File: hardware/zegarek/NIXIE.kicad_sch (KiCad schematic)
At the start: 42 parts, among them M1 74141DIP16, M2 74141DIP16, M3 74141DIP16, M4 74141DIP16, U5 SN74LVC8T245, U6 SN74LVC8T245

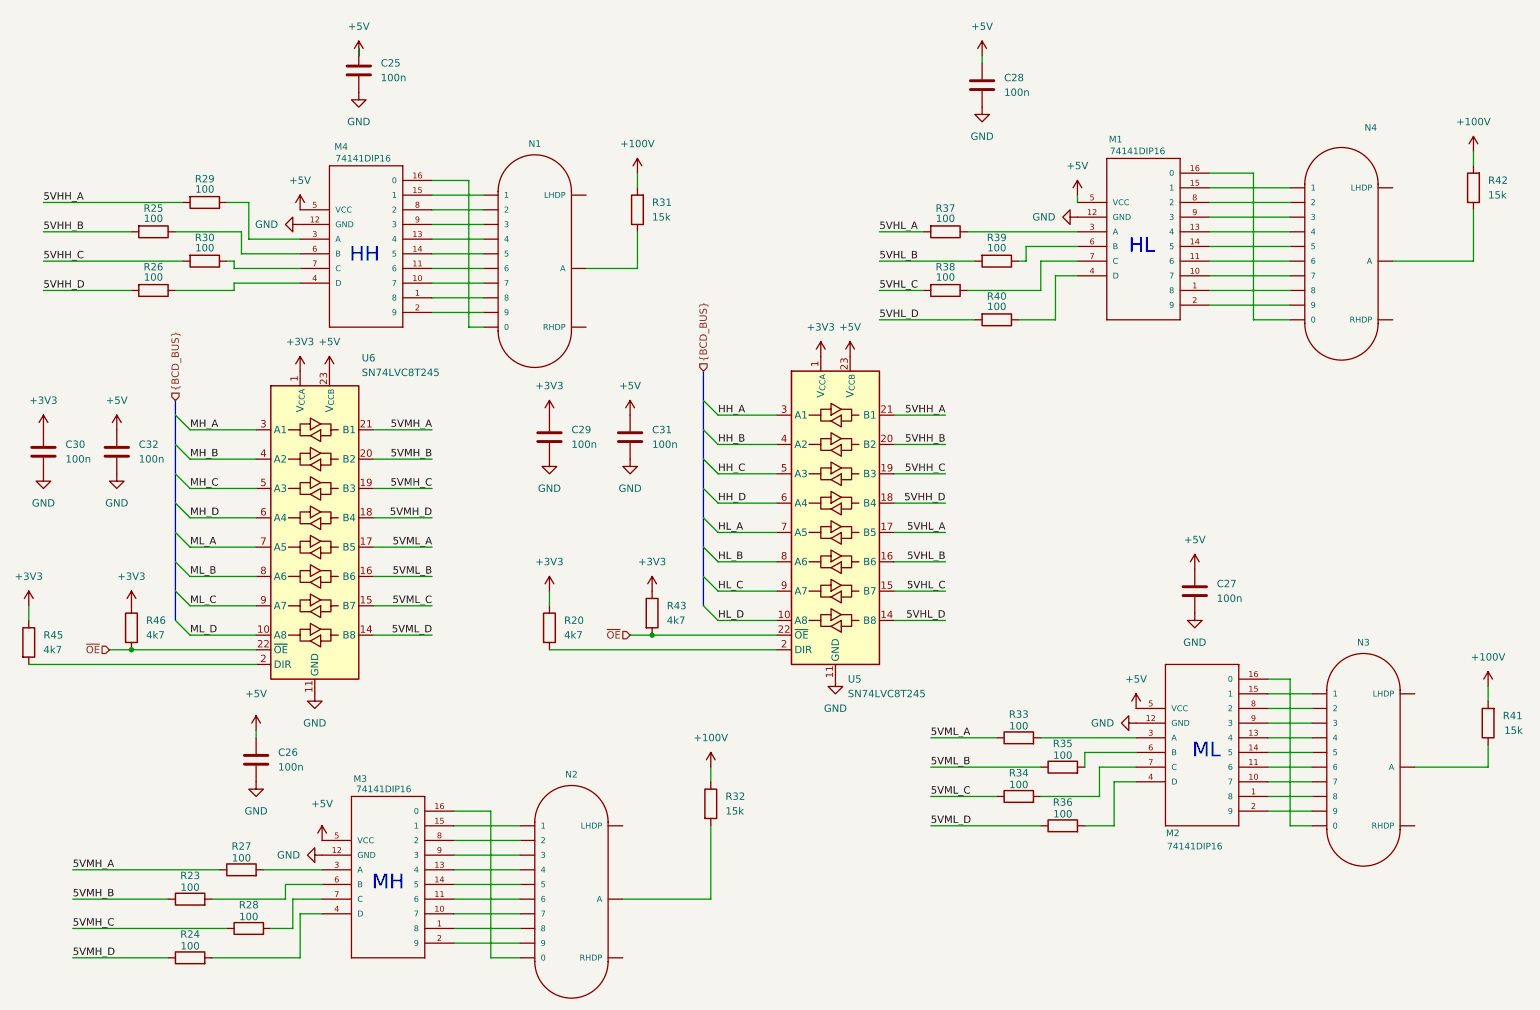
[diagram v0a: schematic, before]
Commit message: reqenerating postprod
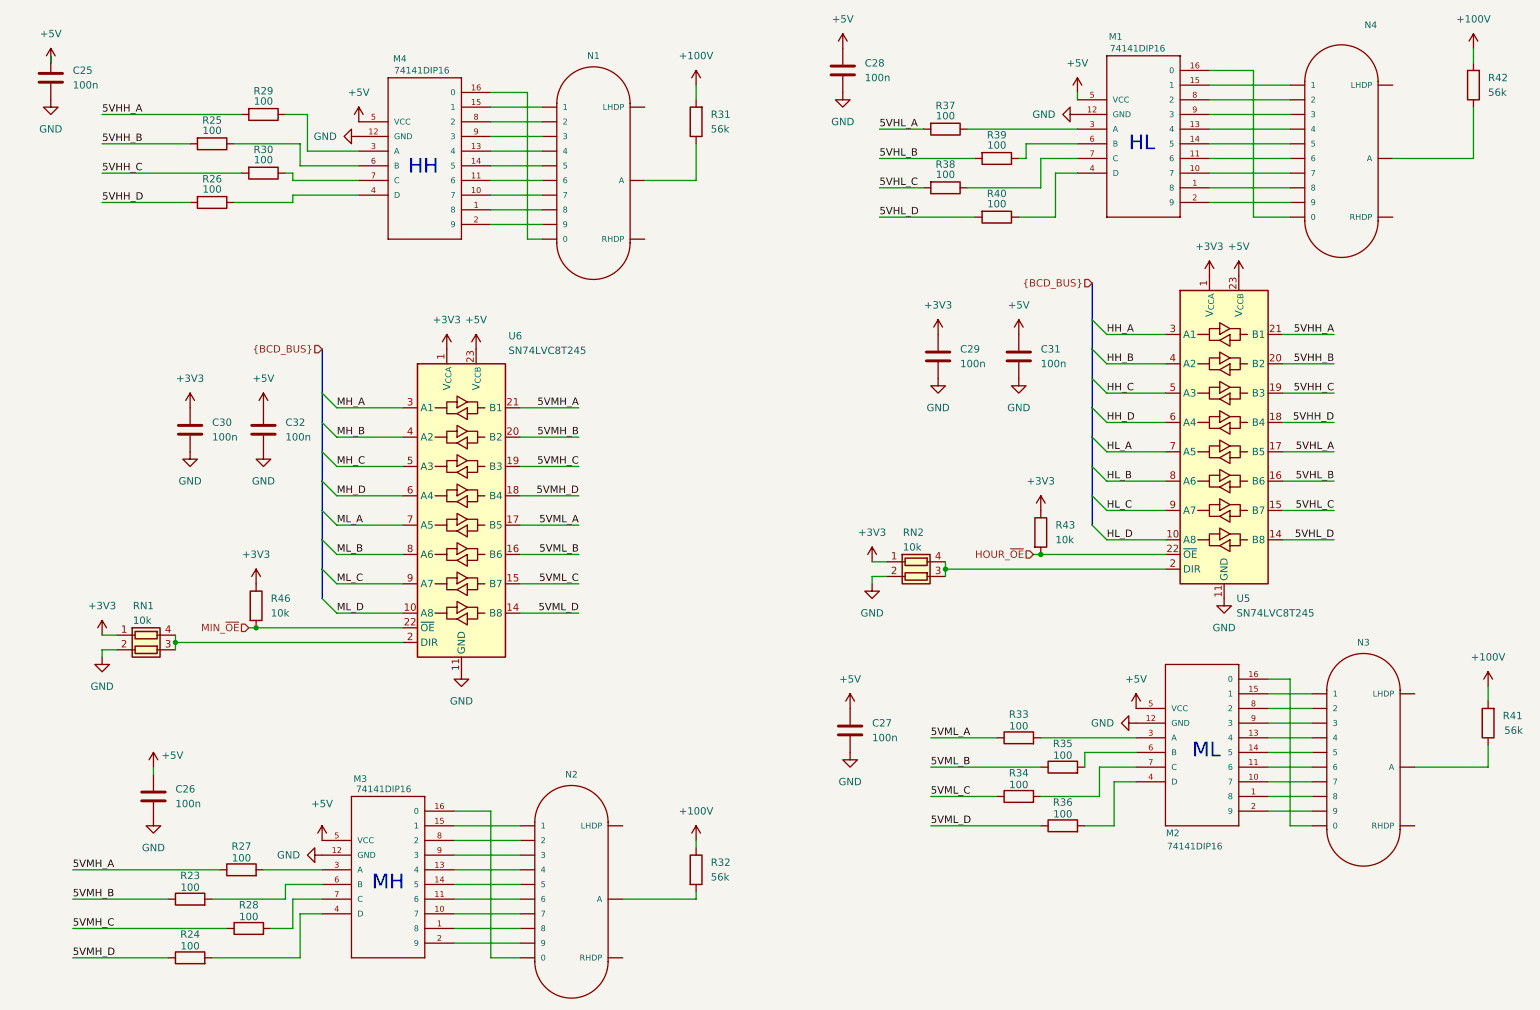
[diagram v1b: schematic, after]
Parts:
- removed R20, R45: 4k7, symbol Device:R
- added RN1, RN2: 10k, Resistor_SMD:R_Array_Convex_2x0606, symbol Device:R_Pack02
- R31, R32, R41, R42: value 15k -> 56k; footprint Resistor_SMD:R_0603_1608Metric_Pad0.98x0.95mm_HandSolder -> Resistor_SMD:R_1206_3216Metric_Pad1.30x1.75mm_HandSolder
- R43, R46: value 4k7 -> 10k; footprint (none) -> Resistor_SMD:R_0603_1608Metric_Pad0.98x0.95mm_HandSolder
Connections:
- net +3V3: now also RN1.1 (R1.1), RN2.1 (R1.1)
- net GND: now also RN1.2 (R2.1), RN2.2 (R2.1)
- net at U5.2 (DIR): now also RN2.3 (R2.2), RN2.4 (R1.2)
- net at U6.2 (DIR): now also RN1.3 (R2.2), RN1.4 (R1.2)
- net ~{OE} renamed HOUR_~{OE}
- net HOUR_~{OE}: no longer R46.2, U6.22 (~{OE})
- new net MIN_~{OE}: R46.2, U6.22 (~{OE})
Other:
- moved on the sheet: C25, C26, C27, C28, C29, C30, C31, C32, M1, M4, N1, N4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
